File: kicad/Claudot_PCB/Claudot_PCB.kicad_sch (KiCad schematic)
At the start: 47 parts, among them SW1 SW_Push, SW10 SW_Push, SW11 SW_Push, SW12 RotaryEncoder, SW2 SW_Push, SW3 SW_Push, SW4 SW_Push, SW5 SW_Push, SW6 SW_Push, SW7 SW_Push, SW8 SW_Push, SW9 SW_Push, U1 RP2040, U2 AP2112K-3.3, U3 W25Q16JVUXIQ, Y1 12MHz

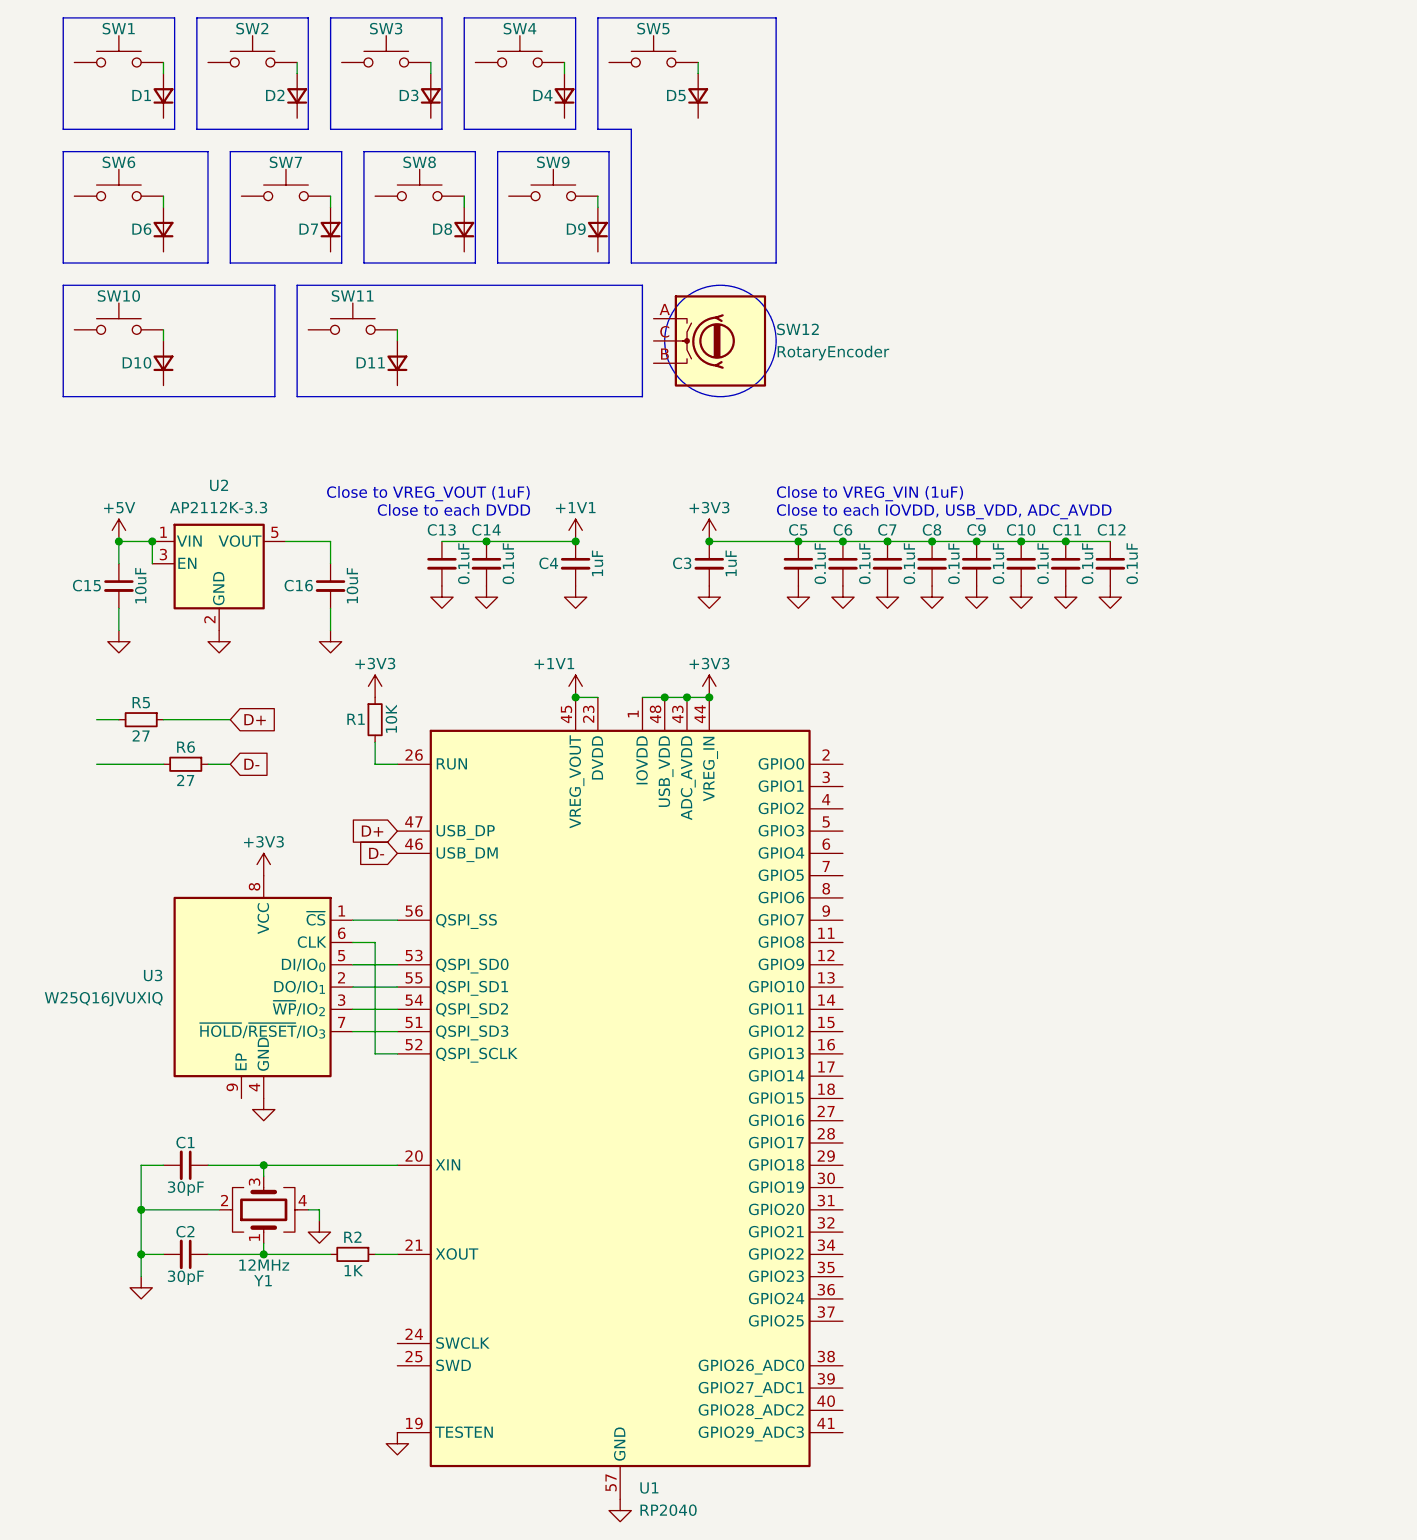
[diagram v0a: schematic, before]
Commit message: Update schematic and pcb
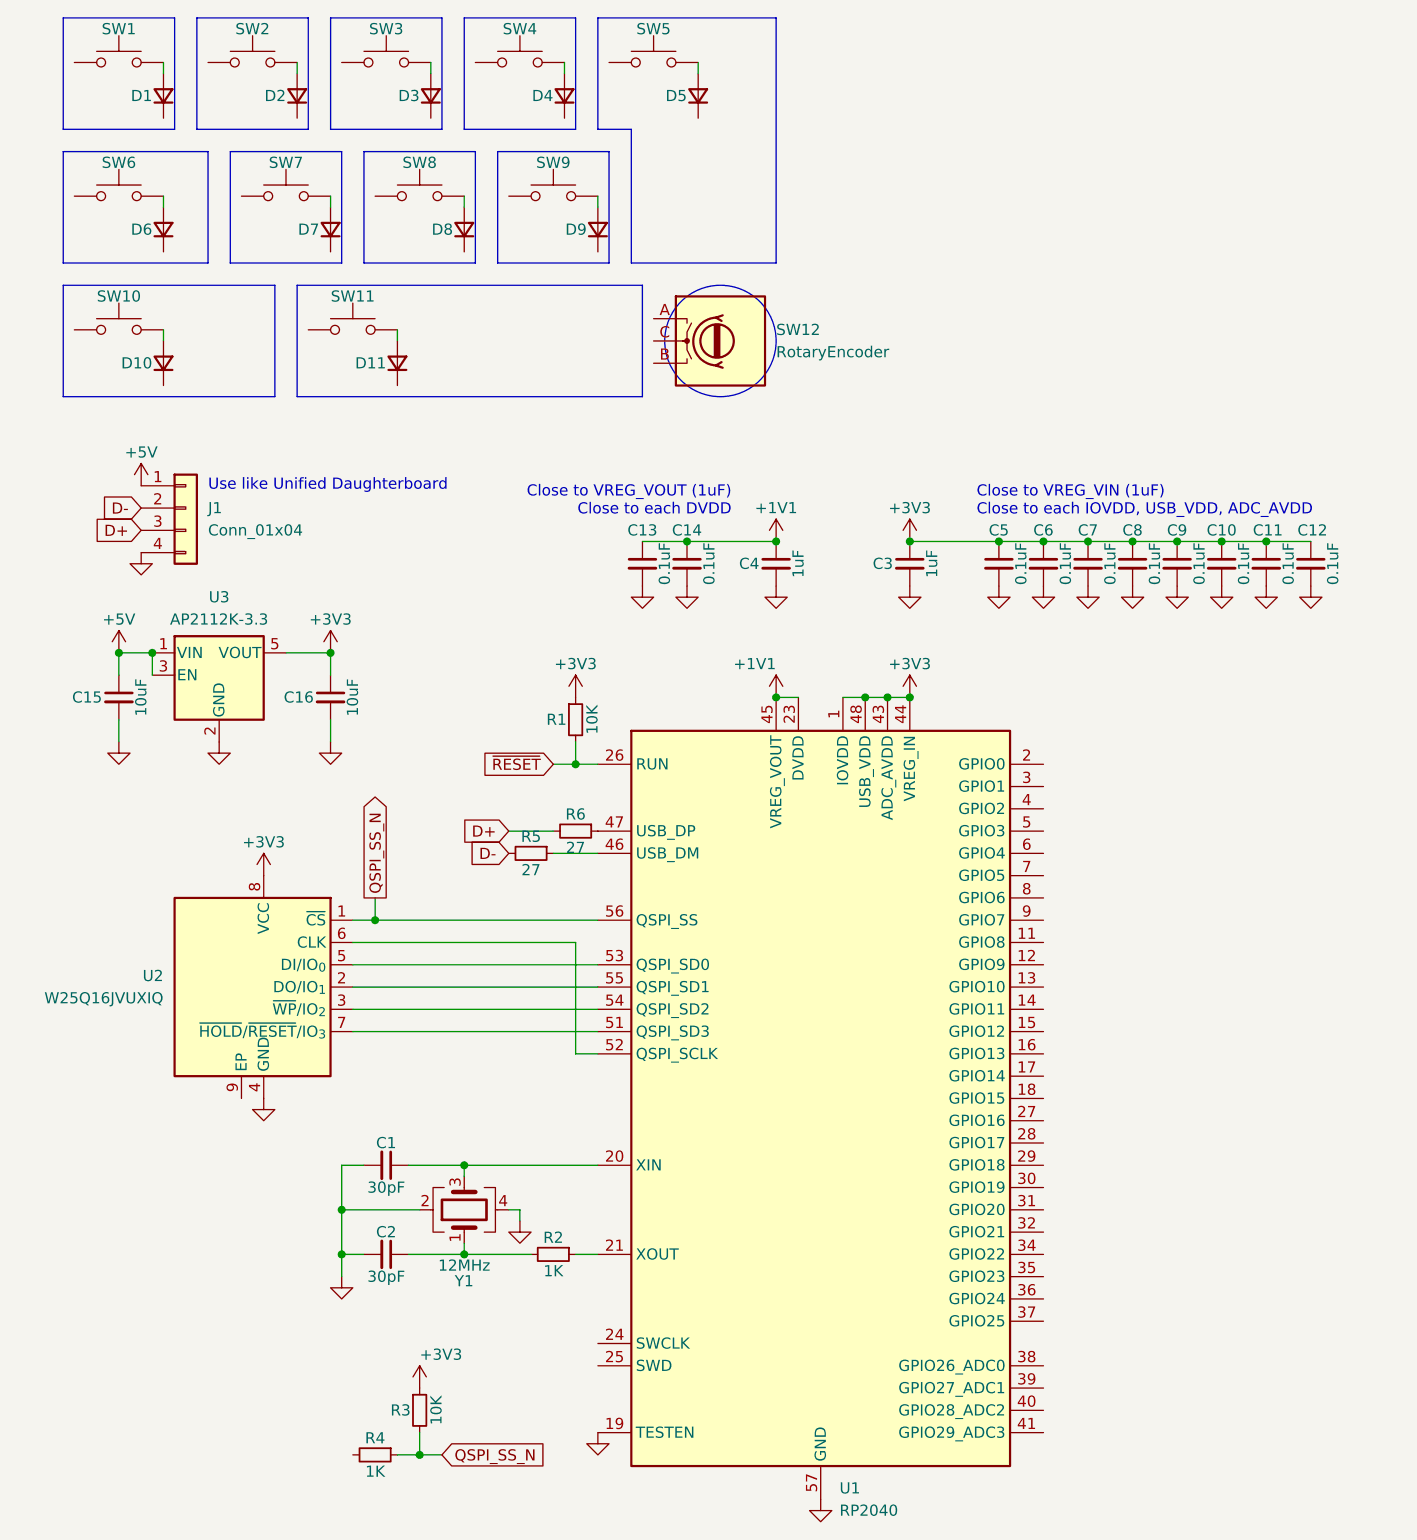
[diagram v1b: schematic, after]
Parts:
- added J1: Conn_01x04, Connector_Molex:Molex_Pico-EZmate_78171-0004_1x04-1MP_P1.20mm_Vertical, symbol Connector_Generic:Conn_01x04
- added R3: 10K, Resistor_SMD:R_0402_1005Metric, symbol Device:R_Small
- added R4: 1K, Resistor_SMD:R_0402_1005Metric, symbol Device:R_Small
- renumbered U3 to U2, U2 to U3
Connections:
- net +3V3: now also C16.1, U3.5 (VOUT), R3.1
- net +5V: now also J1.1 (Pin_1)
- net D+: now also R6.2, J1.3 (Pin_3); no longer R5.1, U1.47 (USB_DP)
- net D-: now also R5.2, J1.2 (Pin_2); no longer R6.1, U1.46 (USB_DM)
- net GND: now also J1.4 (Pin_4)
- net QSPI_SS_N: now reaches U1.56 (QSPI_SS), U2.1 (~{CS})
- net QSPI_SS_N: now also R3.2, R4.1
- net ~{RESET}: now reaches R1.2, U1.26 (RUN)
- new net: R6.1, U1.47 (USB_DP)
- new net: R5.1, U1.46 (USB_DM)
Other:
- note added: "Use like Unified Daughterboard"
- moved on the sheet: C1, C10, C11, C12, C13, C14, C15, C16, C2, C3, C4, C5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
